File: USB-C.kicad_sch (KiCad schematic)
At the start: 22 parts, among them IC2 TPS2557QDRBTQ1, IC5 TPS2557QDRBTQ1, J4 USB_C_Receptacle, J5 USB_C_Receptacle_USB2.0_16P

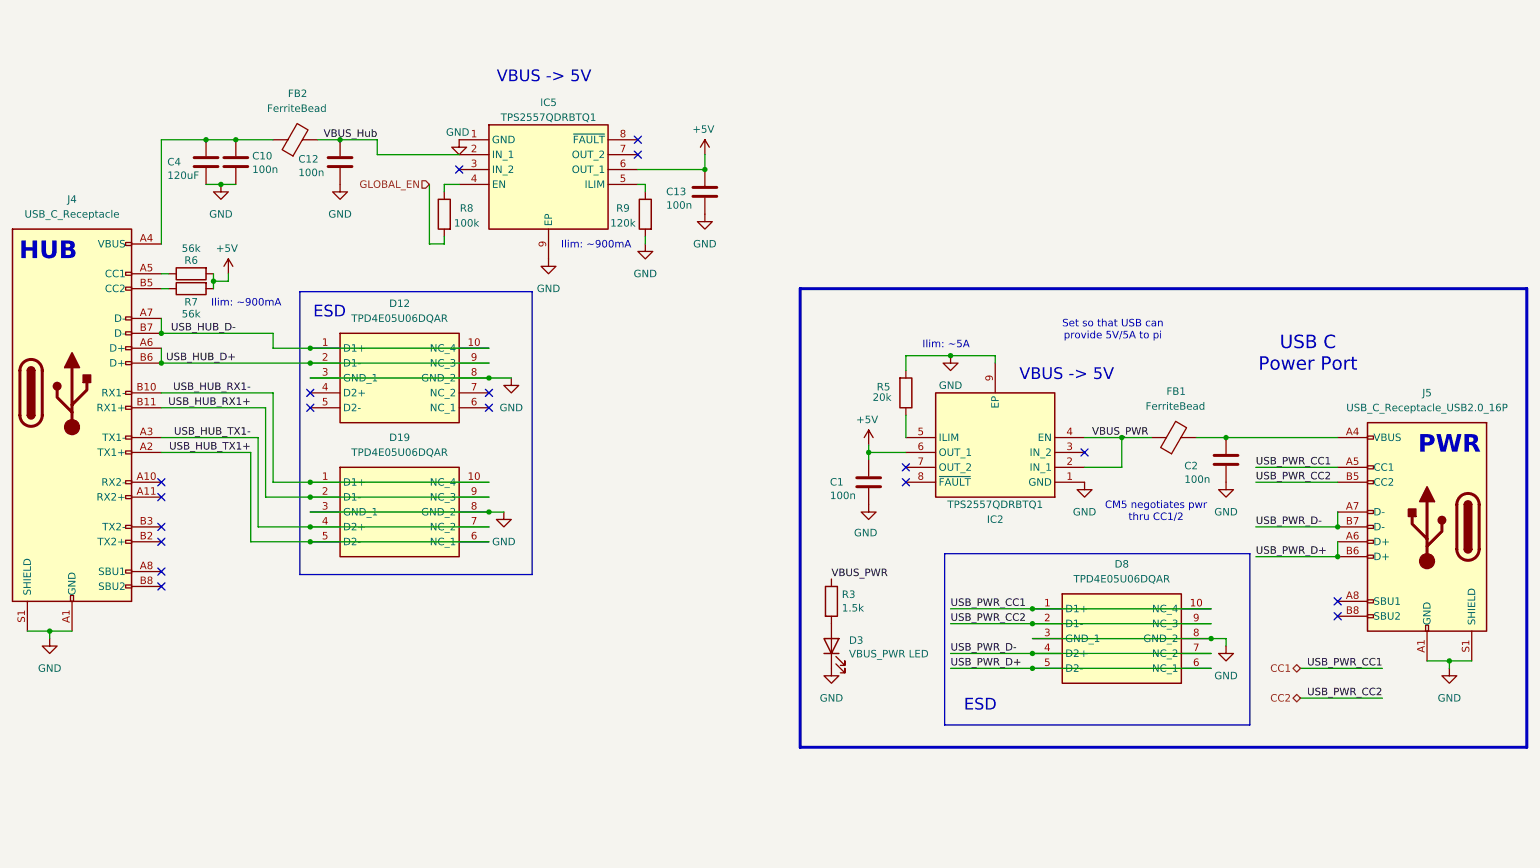
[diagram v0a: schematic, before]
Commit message: rrrrrrrr
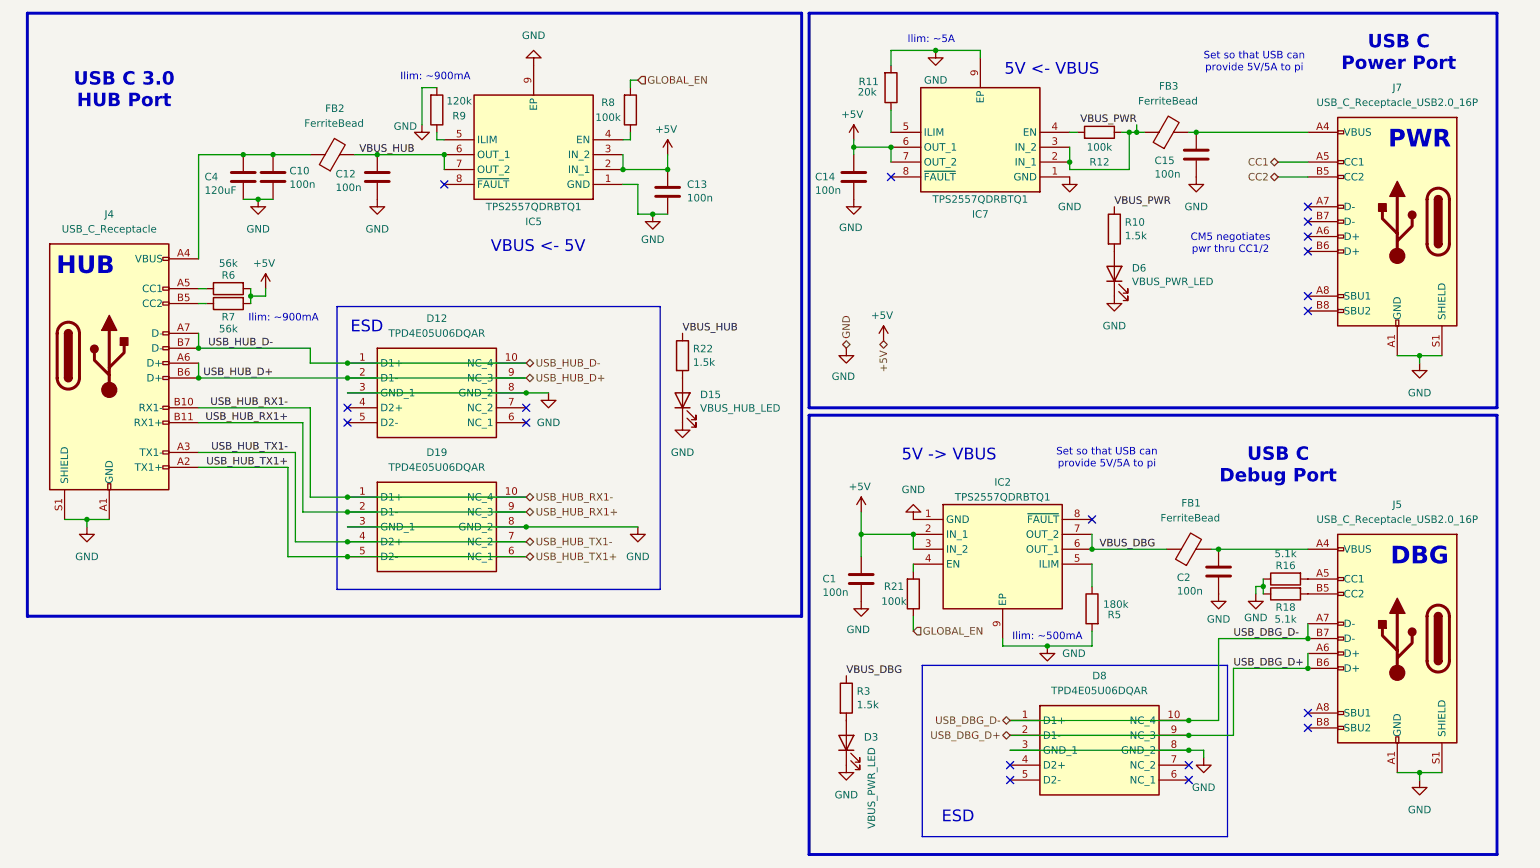
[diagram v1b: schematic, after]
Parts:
- added C14, C15: 100n, Capacitor_SMD:C_0603_1608Metric, symbol Device:C
- added D15: VBUS_HUB_LED, LED_SMD:LED_0603_1608Metric, symbol Device:LED
- added D6: VBUS_PWR_LED, LED_SMD:LED_0603_1608Metric, symbol Device:LED
- added FB3: FerriteBead, Inductor_SMD:L_1206_3216Metric, symbol Device:FerriteBead
- added IC7: TPS2557QDRBTQ1, SON65P300X300X100-9N-D, symbol TPS2557QDRBTQ1:TPS2557QDRBTQ1
- added J7: USB_C_Receptacle_USB2.0_16P, Connector_USB:USB_C_Receptacle_GCT_USB4105-xx-A_16P_TopMnt_Horizontal, symbol Connector:USB_C_Receptacle_USB2.0_16P
- added R10, R22: 1.5k, Resistor_SMD:R_0603_1608Metric, symbol Device:R
- added R11: 20k, Resistor_SMD:R_0603_1608Metric, symbol Device:R
- added R12, R21: 100k, Resistor_SMD:R_0603_1608Metric, symbol Device:R
- added R16, R18: 5.1k, Resistor_SMD:R_0603_1608Metric, symbol Device:R
- D3: value VBUS_PWR LED -> VBUS_PWR_LED
- R5: value 20k -> 180k
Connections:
- net +5V: now also IC2.2 (IN_1), IC2.3 (IN_2), IC5.2 (IN_1), IC5.3 (IN_2), C14.1, IC7.6 (OUT_1), IC7.7 (OUT_2); no longer IC2.6 (OUT_1), IC5.6 (OUT_1)
- net CC1: now also J7.A5 (CC1); no longer D8.1 (D1+), D8.10 (NC_4), J5.A5 (CC1)
- net CC2: now also J7.B5 (CC2); no longer D8.2 (D1-), D8.9 (NC_3), J5.B5 (CC2)
- net GLOBAL_EN: now also R21.1
- net GND: now also C14.2, C15.2, D15.1 (K), D6.1 (K), IC7.1 (GND), IC7.9 (EP), J7.A1 (GND), J7.A12 (GND), J7.B1 (GND), J7.B12 (GND), J7.S1 (SHIELD), R11.2, R16.1, R18.1
- net VBUS_PWR: now also FB3.1, IC7.2 (IN_1), IC7.3 (IN_2), R10.1, R12.1; no longer FB1.1, IC2.2 (IN_1), IC2.4 (EN), R3.1
- net VBUS_HUB: now reaches IC5.7 (OUT_2)
- net VBUS_HUB: now also C12.1, FB2.2, IC5.6 (OUT_1), R22.1
- net VBUS_DBG: now reaches IC2.7 (OUT_2)
- net VBUS_DBG: now also FB1.1, IC2.6 (OUT_1), R3.1
- net USB_PWR_D+ renamed USB_DBG_D+
- net USB_DBG_D+: now also D8.2 (D1-), D8.9 (NC_3); no longer D8.5 (D2-), D8.6 (NC_1)
- net USB_PWR_D- renamed USB_DBG_D-
- net USB_DBG_D-: now also D8.1 (D1+), D8.10 (NC_4); no longer D8.4 (D2+), D8.7 (NC_2)
- removed net VBUS_Hub: C12.1, FB2.2, IC5.2 (IN_1)
- new net: D6.2 (A), R10.2
- new net: C15.1, FB3.2, J7.A4 (VBUS), J7.A9 (VBUS), J7.B4 (VBUS), J7.B9 (VBUS)
- new net: IC2.4 (EN), R21.2
- new net: IC7.4 (EN), R12.2
- new net: J5.A5 (CC1), R16.2
- new net: IC7.5 (ILIM), R11.1
- new net: D15.2 (A), R22.2
- new net: J5.B5 (CC2), R18.2
- no-connect marks 18 -> 19
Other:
- note added: "5V -> VBUS"
- note added: "5V <- VBUS"
- note added: "DBG"
- note added: "Ilim: ~500mA"
- note added: "USB C 3.0 HUB Port"
- note added: "USB C Debug Port"
- note added: "VBUS <- 5V"
- note removed: "VBUS -> 5V"
- moved on the sheet: C1, C10, C12, C2, C4, D12, D19, D3, D8, FB1, FB2, IC2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

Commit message: Schem done? [plz full review], redoing layout
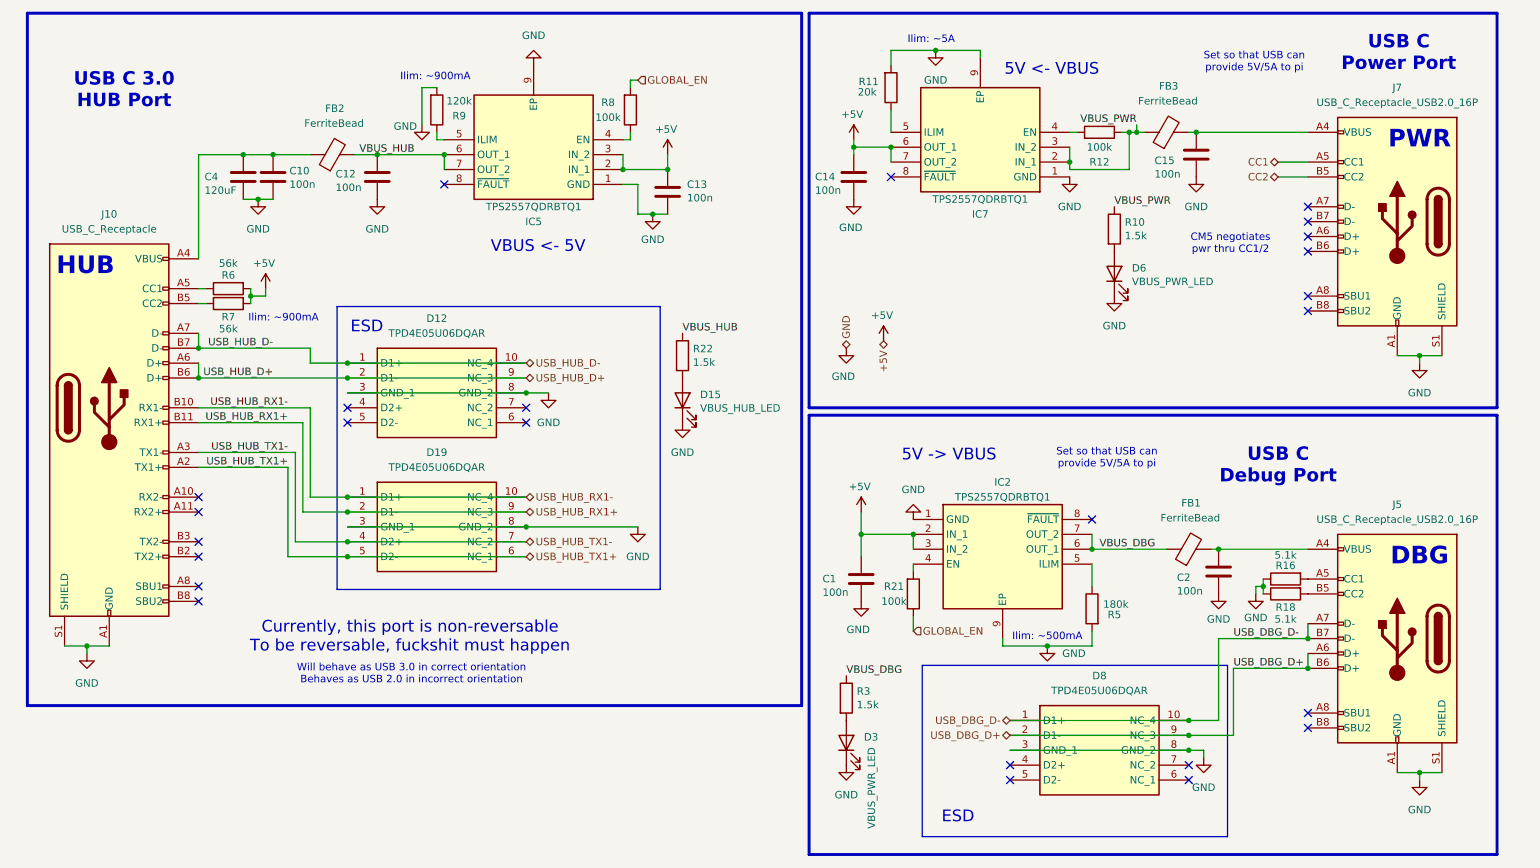
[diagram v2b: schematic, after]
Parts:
- removed J4: USB_C_Receptacle, symbol Connector:USB_C_Receptacle
- added J10: USB_C_Receptacle, Connector_USB:USB_C_Receptacle_Molex_105450-0101, symbol Connector:USB_C_Receptacle
- D12, D19, D8: footprint Controls_Pi:DQA_R-PUSON-N10_ -> Controls_Pi:IC_TPD4E05U06QDQARQ1
- IC2, IC5, IC7: footprint SON65P300X300X100-9N-D -> Controls_Pi:SON65P300X300X100-9N-D
- J7: footprint Connector_USB:USB_C_Receptacle_GCT_USB4105-xx-A_16P_TopMnt_Horizontal -> UTSVT_Connectors:USB_C_Receptacle_GCT_USB4105-xx-A_16P_TopMnt_Horizontal
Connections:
- net GND: now also J10.A1 (GND), J10.A12 (GND), J10.B1 (GND), J10.B12 (GND), J10.S1 (SHIELD)
- net USB_HUB_D+: now also J10.A6 (D+), J10.B6 (D+)
- net USB_HUB_D-: now also J10.A7 (D-), J10.B7 (D-)
- net USB_HUB_RX1+: now also J10.B11 (RX1+)
- net USB_HUB_RX1-: now also J10.B10 (RX1-)
- net USB_HUB_TX1+: now also J10.A2 (TX1+)
- net USB_HUB_TX1-: now also J10.A3 (TX1-)
- net at C10.1, C4.1, FB2.1: now also J10.A4 (VBUS), J10.A9 (VBUS), J10.B4 (VBUS), J10.B9 (VBUS)
- net at R7.1: now also J10.B5 (CC2)
- net at R6.1: now also J10.A5 (CC1)
- no-connect marks 19 -> 25
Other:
- note added: "Currently, this port is non-reversable To be reversable, fuckshit must happen"
- note added: "Will behave as USB 3.0 in correct orientation Behaves as USB 2.0 in incorrect orientation"
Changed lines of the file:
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@@
 	(rectangle
 		(start 22.86 15.24)
-		(end 154.94 118.11)
+		(end 154.94 133.35)
 		(stroke
 			(width 0.5)
@@
 		)
 	)
+	(text "Currently, this port is non-reversable\nTo be reversable, fuckshit must happen"
+		(exclude_from_sim no)
+		(at 88.138 121.666 0)
+		(effects
+			(font
+				(size 2 2)
+			)
+		)
+	)
 	(text "5V <- VBUS"
 		(exclude_from_sim no)
@@
 		)
 	)
+	(text "Will behave as USB 3.0 in correct orientation\nBehaves as USB 2.0 in incorrect orientation"
+		(exclude_from_sim no)
+		(at 88.392 128.016 0)
+		(effects
+			(font
+				(size 1.27 1.27)
+			)
+		)
+	)
 	(text "Set so that USB can \nprovide 5V/5A to pi"
 		(exclude_from_sim no)
@@
 	)
 	(junction
-		(at 52.07 72.39)
+		(at 226.06 106.68)
 		(diameter 0)
 		(color 0 0 0 0)
 	)
 	(junction
-		(at 226.06 106.68)
+		(at 220.98 138.43)
 		(diameter 0)
 		(color 0 0 0 0)
 	)
 	(junction
-		(at 220.98 138.43)
+		(at 52.07 72.39)
 		(diameter 0)
 		(color 0 0 0 0)
@@
 	)
 	(junction
-		(at 33.02 101.6)
+		(at 33.02 123.19)
 		(diameter 0)
 		(color 0 0 0 0)
@@
 	)
 	(junction
-		(at 173.99 104.14)
+		(at 52.07 77.47)
 		(diameter 0)
 		(color 0 0 0 0)
 	)
 	(junction
-		(at 260.35 144.78)
+		(at 173.99 104.14)
 		(diameter 0)
 		(color 0 0 0 0)
 	)
 	(junction
-		(at 222.25 35.56)
+		(at 260.35 144.78)
 		(diameter 0)
 		(color 0 0 0 0)
 	)
 	(junction
-		(at 52.07 77.47)
+		(at 222.25 35.56)
 		(diameter 0)
 		(color 0 0 0 0)
@@
 	)
 	(no_connect
+		(at 52.07 105.41)
+	)
+	(no_connect
+		(at 52.07 100.33)
+	)
+	(no_connect
 		(at 241.3 53.34)
 	)
@@
 	)
 	(no_connect
+		(at 52.07 97.79)
+	)
+	(no_connect
+		(at 52.07 113.03)
+	)
+	(no_connect
+		(at 52.07 107.95)
+	)
+	(no_connect
 		(at 204.47 101.6)
 	)
@@
 	)
 	(no_connect
+		(at 52.07 115.57)
+	)
+	(no_connect
 		(at 241.3 63.5)
 	)
@@
 	(wire
 		(pts
-			(xy 33.02 101.6) (xy 33.02 102.87)
+			(xy 33.02 123.19) (xy 33.02 124.46)
 		)
 		(stroke
@@
 	(wire
 		(pts
-			(xy 29.21 101.6) (xy 33.02 101.6)
+			(xy 29.21 123.19) (xy 33.02 123.19)
 		)
 		(stroke
@@
 	(wire
 		(pts
-			(xy 33.02 101.6) (xy 36.83 101.6)
+			(xy 33.02 123.19) (xy 36.83 123.19)
 		)
 		(stroke
@@
 			)
 		)
-		(property "Footprint" "SON65P300X300X100-9N-D"
+		(property "Footprint" "Controls_Pi:SON65P300X300X100-9N-D"
 			(at 97.79 -50.47 0)
 			(effects
@@
 			)
 		)
-		(property "Footprint" "Controls_Pi:DQA_R-PUSON-N10_"
+		(property "Footprint" "Controls_Pi:IC_TPD4E05U06QDQARQ1"
 			(at 104.14 169.85 0)
 			(effects
@@
 		)
 		(property "Value" "5.1k"
-			(at 237.49 107.442 90)
+			(at 237.49 107.696 90)
 			(effects
 				(font
@@
 	)
 	(symbol
-		(lib_id "Connector:USB_C_Receptacle")
-		(at 36.83 82.55 0)
-		(unit 1)
-		(exclude_from_sim no)
-		(in_bom yes)
-		(on_board yes)
-		(dnp no)
-		(fields_autoplaced yes)
-		(property "Reference" "J4"
-			(at 36.83 49.53 0)
-			(effects
-				(font
-					(size 1.27 1.27)
-				)
-			)
-		)
-		(property "Value" "USB_C_Receptacle"
-			(at 36.83 52.07 0)
-			(effects
-				(font
-					(size 1.27 1.27)
-				)
-			)
-		)
-		(property "Footprint" ""
-			(at 40.64 82.55 0)
-			(effects
-				(font
-					(size 1.27 1.27)
-				)
-				(hide yes)
-			)
-		)
-		(property "Datasheet" "https://www.usb.org/sites/default/files/documents/usb_type-c.zip"
-			(at 40.64 82.55 0)
-			(effects
-				(font
-					(size 1.27 1.27)
-				)
-				(hide yes)
-			)
-		)
-		(property "Description" "USB Full-Featured Type-C Receptacle connector"
-			(at 36.83 82.55 0)
-			(effects
-				(font
-					(size 1.27 1.27)
-				)
-				(hide yes)
-			)
-		)
-		(pin "S1"
-		)
-		(pin "A2"
-		)
-		(pin "B4"
-		)
-		(pin "B7"
-		)
-		(pin "B12"
-		)
-		(pin "A1"
-		)
-		(pin "B5"
-		)
-		(pin "A6"
-		)
-		(pin "A3"
-		)
-		(pin "A4"
-		)
-		(pin "B1"
-		)
-		(pin "B10"
-		)
-		(pin "A9"
-		)
-		(pin "B9"
-		)
-		(pin "B6"
-		)
-		(pin "B11"
-		)
-		(pin "A12"
-		)
-		(pin "A5"
-		)
-		(pin "A7"
-		)
-		(instances
-			(project "PiBoard"
-				(path "/e4d65698-b8ec-4bf6-9f2b-a5010377155a/2dec5fd6-8756-425d-9ae9-2f1c2fc4e6c1/65247ae0-83ec-4f51-af4d-84b2c055b0d6"
-					(reference "J4")
-					(unit 1)
-				)
-			)
-		)
-	)
-	(symbol
 		(lib_id "power:GND")
 		(at 177.8 21.59 0)
@@
 			)
 		)
-		(property "Footprint" "Controls_Pi:DQA_R-PUSON-N10_"
+		(property "Footprint" "Controls_Pi:IC_TPD4E05U06QDQARQ1"
 			(at 217.17 230.81 0)
 			(effects
@@
 	)
 	(symbol
+		(lib_name "USB_C_Receptacle_1")
+		(lib_id "Connector:USB_C_Receptacle")
+		(at 36.83 82.55 0)
+		(unit 1)
+		(exclude_from_sim no)
+		(in_bom yes)
+		(on_board yes)
+		(dnp no)
+		(fields_autoplaced yes)
+		(property "Reference" "J10"
+			(at 36.83 49.53 0)
+			(effects
+				(font
+					(size 1.27 1.27)
+				)
+			)
+		)
+		(property "Value" "USB_C_Receptacle"
+			(at 36.83 52.07 0)
+			(effects
+				(font
+					(size 1.27 1.27)
+				)
+			)
+		)
+		(property "Footprint" "Connector_USB:USB_C_Receptacle_Molex_105450-0101"
+			(at 40.64 82.55 0)
+			(effects
+				(font
+					(size 1.27 1.27)
+				)
+				(hide yes)
+			)
+		)
+		(property "Datasheet" "https://www.usb.org/sites/default/files/documents/usb_type-c.zip"
+			(at 40.64 82.55 0)
+			(effects
+				(font
+					(size 1.27 1.27)
+				)
+				(hide yes)
+			)
+		)
+		(property "Description" "USB Full-Featured Type-C Receptacle connector"
+			(at 36.83 82.55 0)
+			(effects
+				(font
+					(size 1.27 1.27)
+				)
+				(hide yes)
+			)
+		)
+		(property "P/N" "105450-0101"
+			(at 36.83 82.55 0)
+			(effects
+				(font
+					(size 1.27 1.27)
+				)
+				(hide yes)
+			)
+		)
+		(pin "B11"
+		)
+		(pin "A1"
+		)
+		(pin "A2"
+		)
+		(pin "A12"
+		)
+		(pin "B12"
+		)
+		(pin "B10"
+		)
+		(pin "A10"
+		)
+		(pin "B9"
+		)
+		(pin "B4"
+		)
+		(pin "B1"
+		)
+		(pin "S1"
+		)
+		(pin "A4"
+		)
+		(pin "B5"
+		)
+		(pin "A7"
+		)
+		(pin "B7"
+		)
+		(pin "A9"
+		)
+		(pin "A5"
+		)
+		(pin "A6"
+		)
+		(pin "B6"
+		)
+		(pin "A3"
+		)
+		(pin "A11"
+		)
+		(pin "B3"
+		)
+		(pin "B2"
+		)
+		(pin "A8"
+		)
+		(pin "B8"
+		)
+		(instances
+			(project ""
+				(path "/e4d65698-b8ec-4bf6-9f2b-a5010377155a/2dec5fd6-8756-425d-9ae9-2f1c2fc4e6c1/65247ae0-83ec-4f51-af4d-84b2c055b0d6"
+					(reference "J10")
+					(unit 1)
+				)
+			)
+		)
+	)
+	(symbol
 		(lib_id "Connector:USB_C_Receptacle_USB2.0_16P")
 		(at 256.54 121.92 0)
@@
 			)
 		)
-		(property "Footprint" "SON65P300X300X100-9N-D"
+		(property "Footprint" "Controls_Pi:SON65P300X300X100-9N-D"
 			(at 173.99 -51.74 0)
 			(effects
@@
 			)
 		)
-		(property "Footprint" "Controls_Pi:DQA_R-PUSON-N10_"
+		(property "Footprint" "Controls_Pi:IC_TPD4E05U06QDQARQ1"
 			(at 104.14 192.71 0)
 			(effects
@@
 			)
 		)
-		(property "Footprint" "SON65P300X300X100-9N-D"
+		(property "Footprint" "Controls_Pi:SON65P300X300X100-9N-D"
 			(at 200.66 196.52 0)
 			(effects
@@
 	(symbol
 		(lib_id "power:GND")
-		(at 33.02 102.87 0)
+		(at 33.02 124.46 0)
 		(unit 1)
 		(exclude_from_sim no)
@@
 		(fields_autoplaced yes)
 		(property "Reference" "#PWR020"
-			(at 33.02 109.22 0)
+			(at 33.02 130.81 0)
 			(effects
 				(font
@@
 		)
 		(property "Value" "GND"
-			(at 33.02 107.95 0)
+			(at 33.02 129.54 0)
 			(effects
 				(font
@@
 		)
 		(property "Footprint" ""
-			(at 33.02 102.87 0)
+			(at 33.02 124.46 0)
 			(effects
 				(font
@@
 		)
 		(property "Datasheet" ""
-			(at 33.02 102.87 0)
+			(at 33.02 124.46 0)
 			(effects
 				(font
@@
 		)
 		(property "Description" "Power symbol creates a global label with name \"GND\" , ground"
-			(at 33.02 102.87 0)
+			(at 33.02 124.46 0)
 			(effects
 				(font
@@
 			)
 		)
-		(property "Footprint" "Connector_USB:USB_C_Receptacle_GCT_USB4105-xx-A_16P_TopMnt_Horizontal"
+		(property "Footprint" "UTSVT_Connectors:USB_C_Receptacle_GCT_USB4105-xx-A_16P_TopMnt_Horizontal"
 			(at 252.73 50.8 0)
 			(effects
